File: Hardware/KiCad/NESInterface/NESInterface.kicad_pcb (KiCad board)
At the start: 2 copper layers, 3.7 x 3.7 mm, 1 part

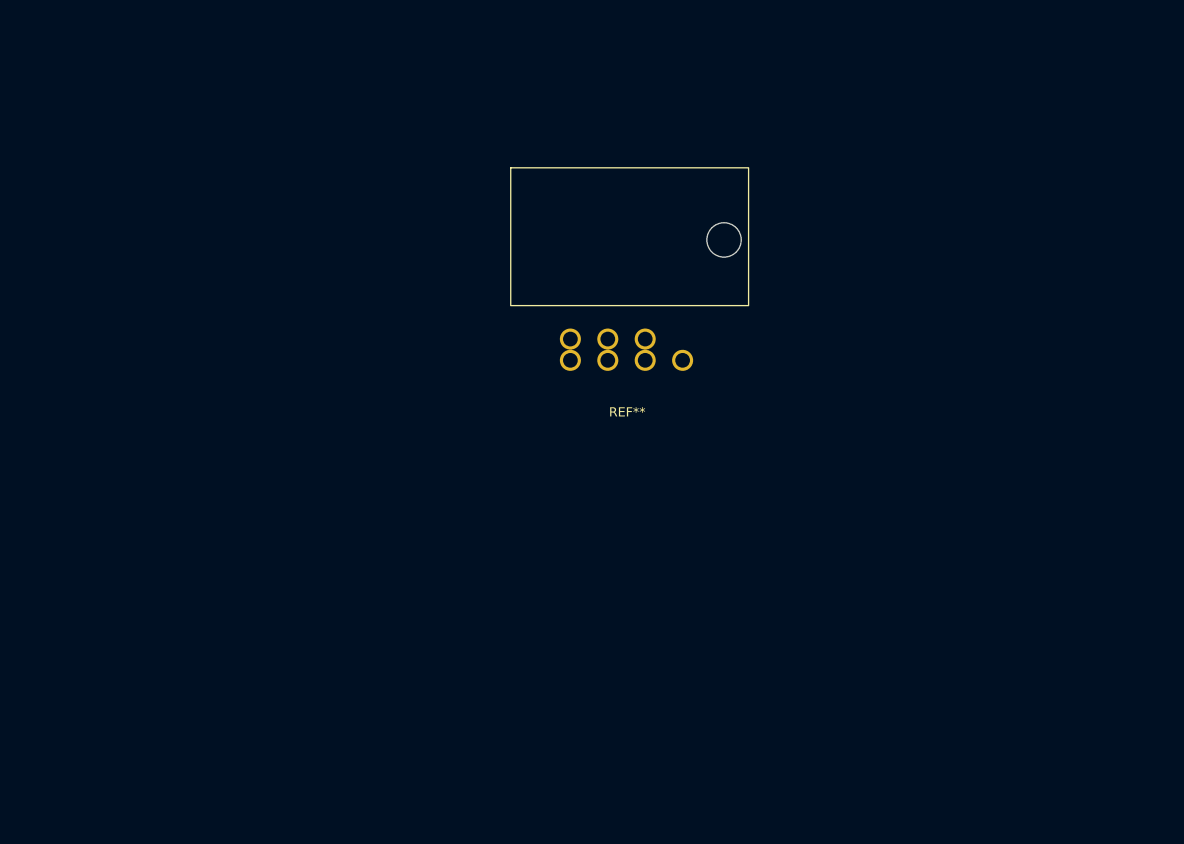
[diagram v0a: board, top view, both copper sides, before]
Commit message: Finished 3D Model
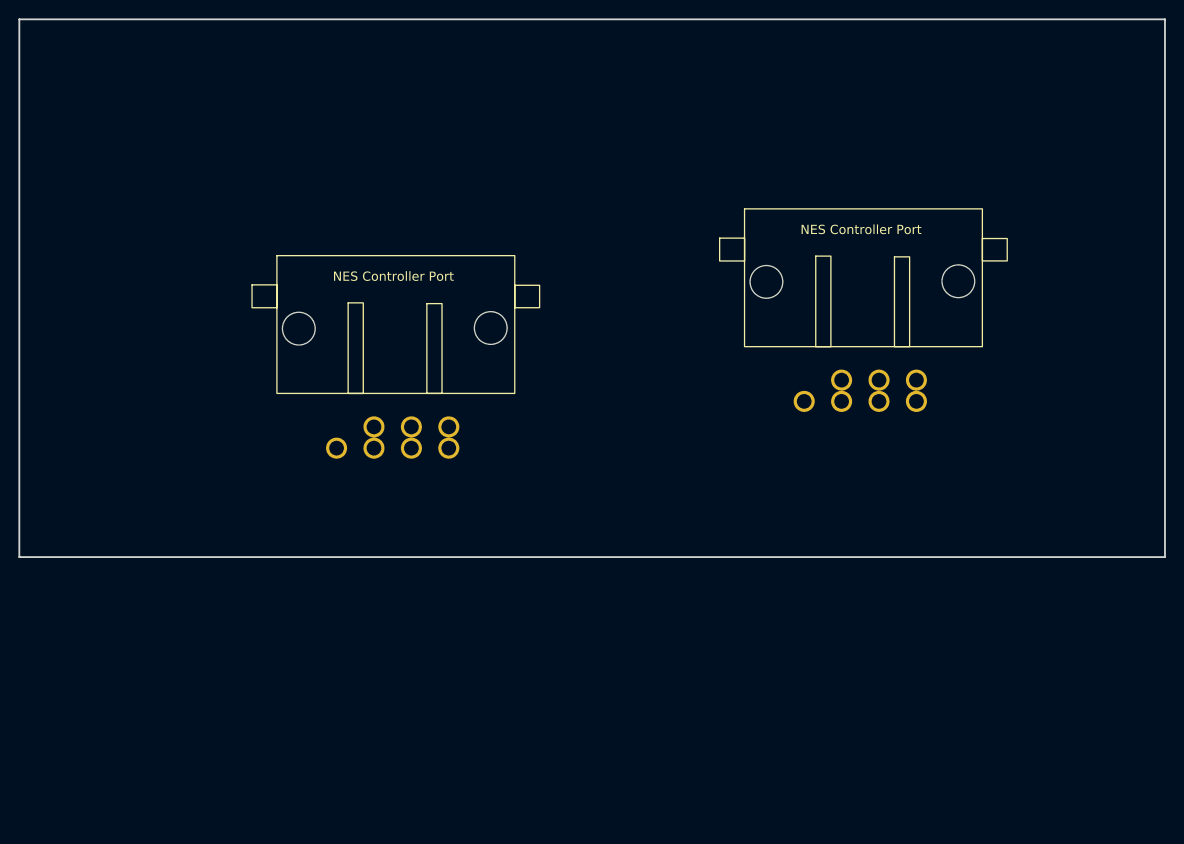
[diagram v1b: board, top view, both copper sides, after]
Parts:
- removed REF**: NES Port, Library:NES Port
- added NES Controller Port: NES Port, Library:NES Port, F.Cu at (66.0, 76.2)
- added NES Controller Port: NES Port, Library:NES Port, F.Cu at (116.8, 71.1)
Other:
- board size 3.7 x 3.7 mm -> 124.5 x 58.4 mm

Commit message: First Rough Board Ordered
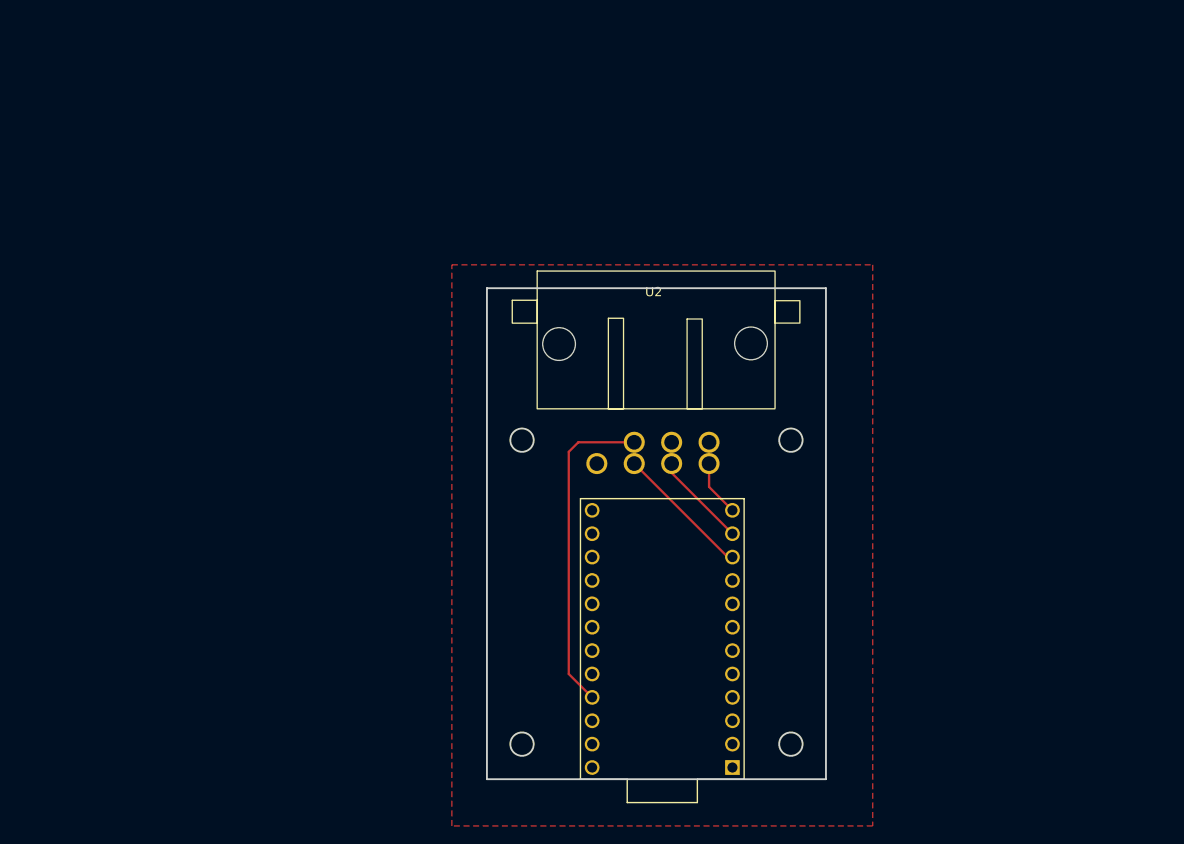
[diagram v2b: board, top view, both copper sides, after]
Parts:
- removed NES Controller Port: NES Port, Library:NES Port (x2)
- added U1: ProMicro, ProMicro:ProMicro, F.Cu at (95.2, 108.0)
- added U2: ~, NES Port:NES Port, F.Cu at (94.3, 77.9)
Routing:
- net VCC: track 0.00 -> 35.3 mm
- net Clock: track 0.00 -> 14.9 mm
- net Latch: track 0.00 -> 10.4 mm
- net Data: track 0.00 -> 6.13 mm
- added copper zone on F.Cu, net GND
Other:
- board size 124.5 x 58.4 mm -> 36.8 x 53.3 mm
- board text added: "Footprint Test Board"
- board text added: "For Project https://github.com/H-Boyd/ NES-controller-USB-interface"
